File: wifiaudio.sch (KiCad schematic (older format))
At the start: 29 parts, among them J1 USB_C_Receptacle_USB2.0, J2 Conn_01x01_Female, J3 Conn_01x01_Female, J4 Conn_01x05_Female, J5 Conn_01x06_Female, J6 Conn_01x01_Female, SW1 SW_DPDT_x2, SW2 SW_Push, U1 ESP-32S, U2 tp4056, U5 ME6211C33M5G-N

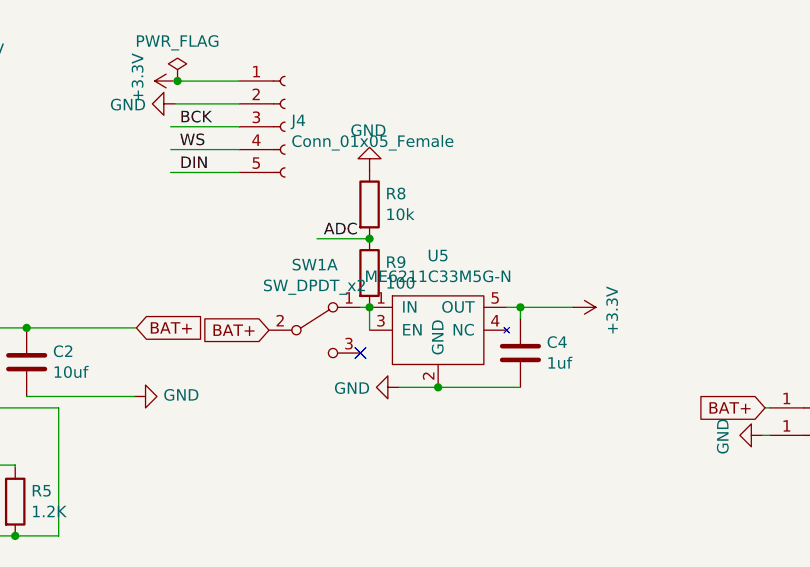
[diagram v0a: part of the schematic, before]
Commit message: 修改readme
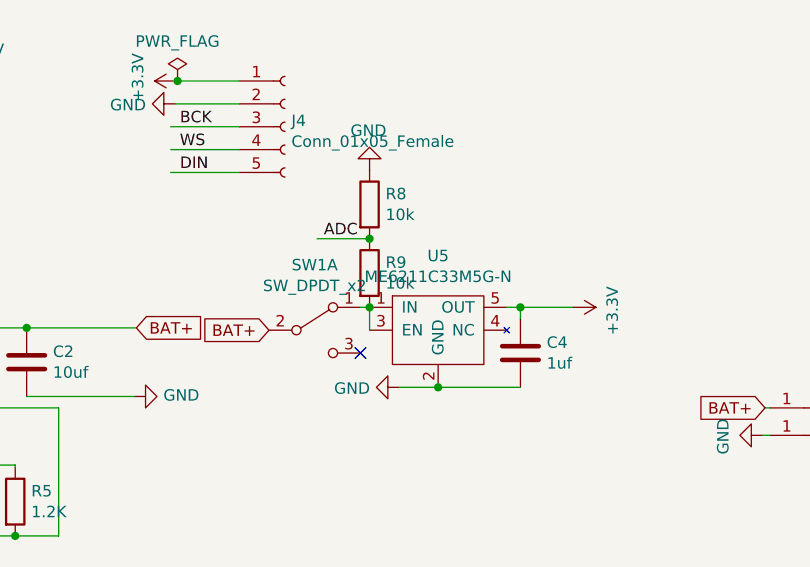
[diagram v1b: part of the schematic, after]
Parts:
- R9: value 100 -> 10k
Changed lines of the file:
@@
 P 6410 4380
 F 0 "R9" H 6480 4426 50  0000 L CNN
-F 1 "100" H 6480 4335 50  0000 L CNN
+F 1 "10k" H 6480 4335 50  0000 L CNN
 F 2 "Resistor_SMD:R_0603_1608Metric" V 6340 4380 50  0001 C CNN
 F 3 "~" H 6410 4380 50  0001 C CNN
